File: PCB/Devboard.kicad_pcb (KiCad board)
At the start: 2 copper layers, 21 x 51 mm, 33 parts, among them J1 USB_C_Receptacle_USB2.0_14P, J2 Conn_01x20, J3 Conn_01x20, J4 Conn_01x03, SW1 SW_Push, U1 RP2040, U2 MCP1700x-330xxTT, U3 W25Q128JVS, Y1 12 MHz

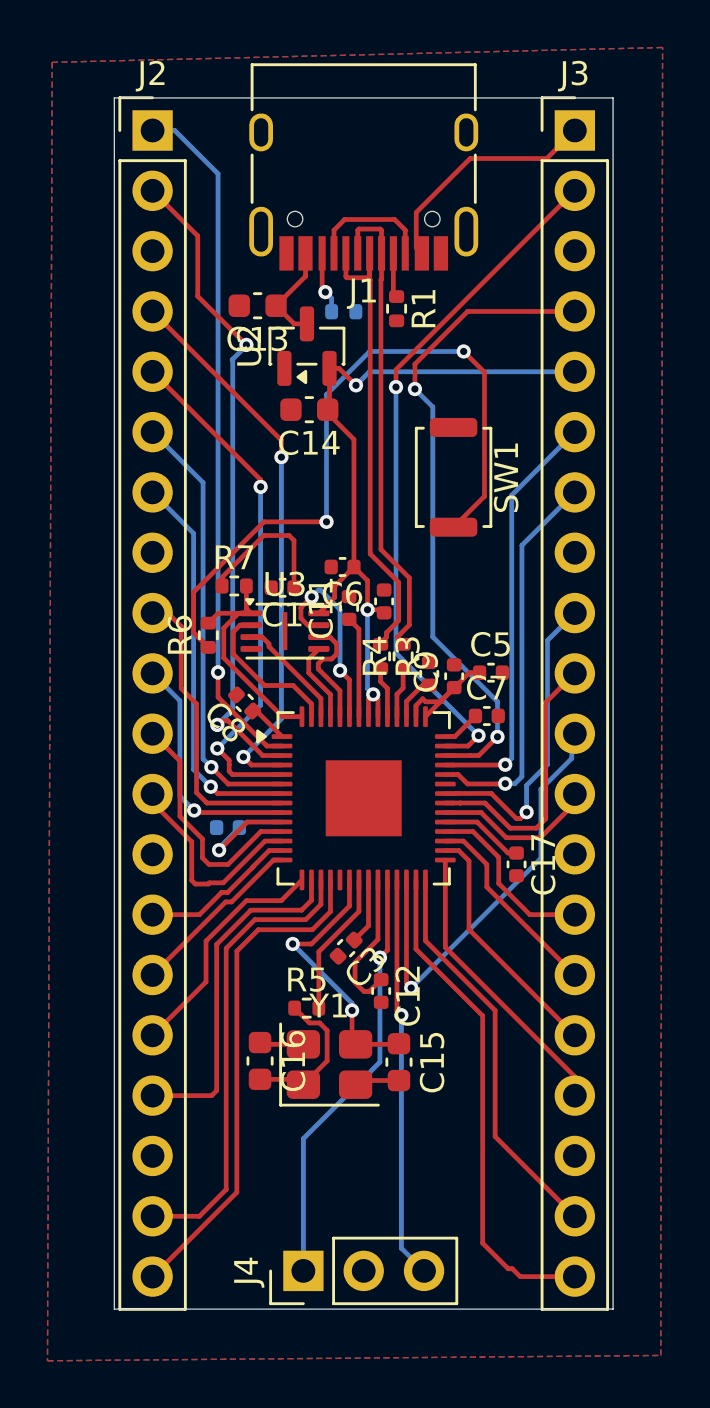
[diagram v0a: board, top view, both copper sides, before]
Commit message: pcb
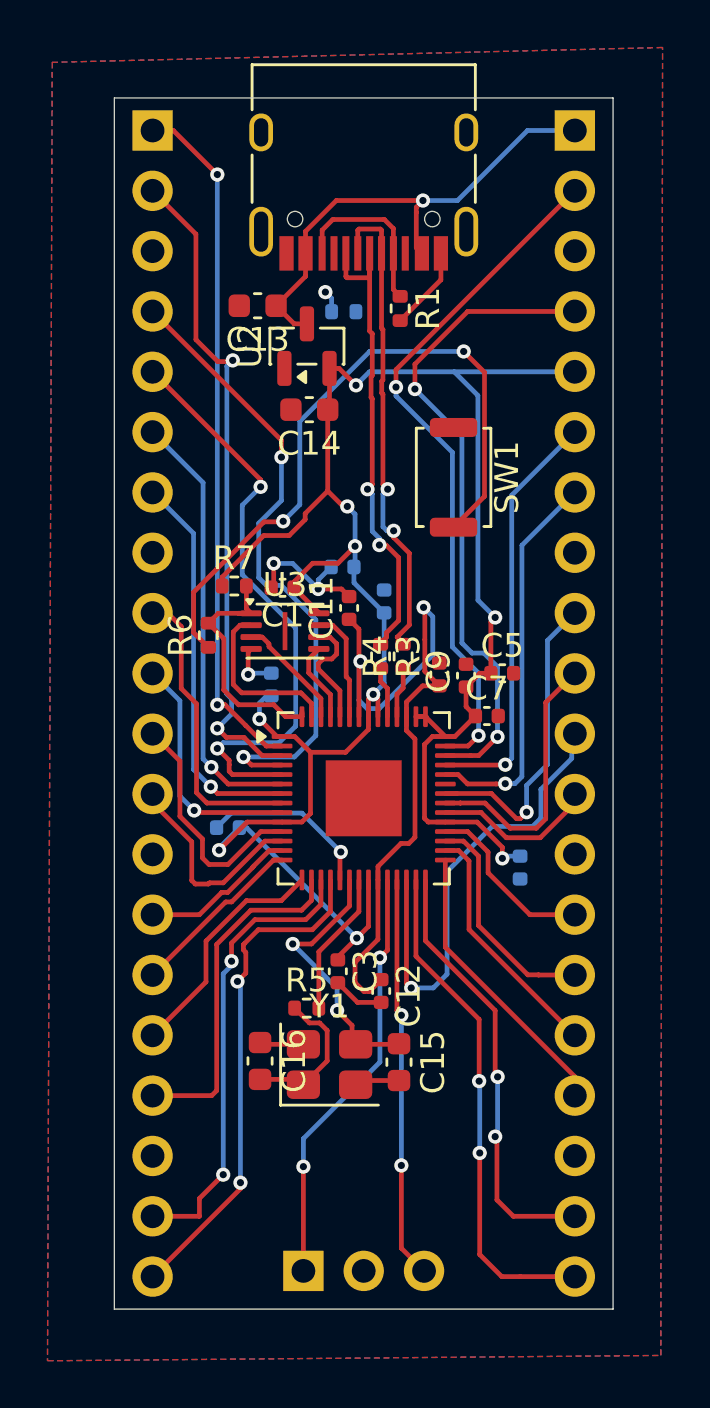
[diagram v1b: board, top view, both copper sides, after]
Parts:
- C17, C4, C6, C8, J2, J3, J4: moved to B.Cu
- moved C8 1.37 mm to (144.5, 99.8), turned to 90 degrees
- moved C3 1.04 mm to (147.3, 111.8), turned to -90 degrees
- moved C9 0.50 mm to (152.7, 99.4)
- moved C5 0.48 mm to (154.2, 99.3)
- moved C10 0.43 mm to (151.6, 99.3)
- moved C17 0.20 mm to (155.0, 107.5)
- moved R1 0.15 mm to (149.9, 83.9)
- turned J2 to 180 degrees
- turned J3 to 180 degrees
- turned J4 to -90 degrees
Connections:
- J1 pad B5: Net-(J1-CC2) -> Net-(J1-CC1)
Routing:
- net +3V3: track 56.6 -> 94.9 mm, vias 4 -> 9
- net GND: track 3.75 -> 24.9 mm, vias 0 -> 4
- net +1V1: track 12.3 -> 32.3 mm, vias 0 -> 2
- net VBUS: track 14.3 -> 20.8 mm, vias 0 -> 1
- net Net-(J1-CC1): track 1.88 -> 7.29 mm
- net (no net): track 5.33 -> 0.00 mm
- net GPIO2: track 23.4 -> 27.1 mm
- net QSPI_SD3: track 8.28 -> 4.73 mm, vias 2 -> 0
- net GPIO3: track 22.0 -> 25.2 mm
- net GPIO17: track 16.8 -> 18.4 mm, vias 0 -> 2
- net RUN: track 18.6 -> 20.2 mm
- net Net-(J1-CC2): track 2.62 -> 1.13 mm
- net GPIO20: track 8.35 -> 9.50 mm
- net Net-(R6-Pad1): track 29.6 -> 28.5 mm
- net GPIO0: track 29.1 -> 30.1 mm, vias 1 -> 2
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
